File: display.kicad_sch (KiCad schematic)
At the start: 53 parts, among them Q3 SSM6N35AFE, Q4 SSM6N35AFE

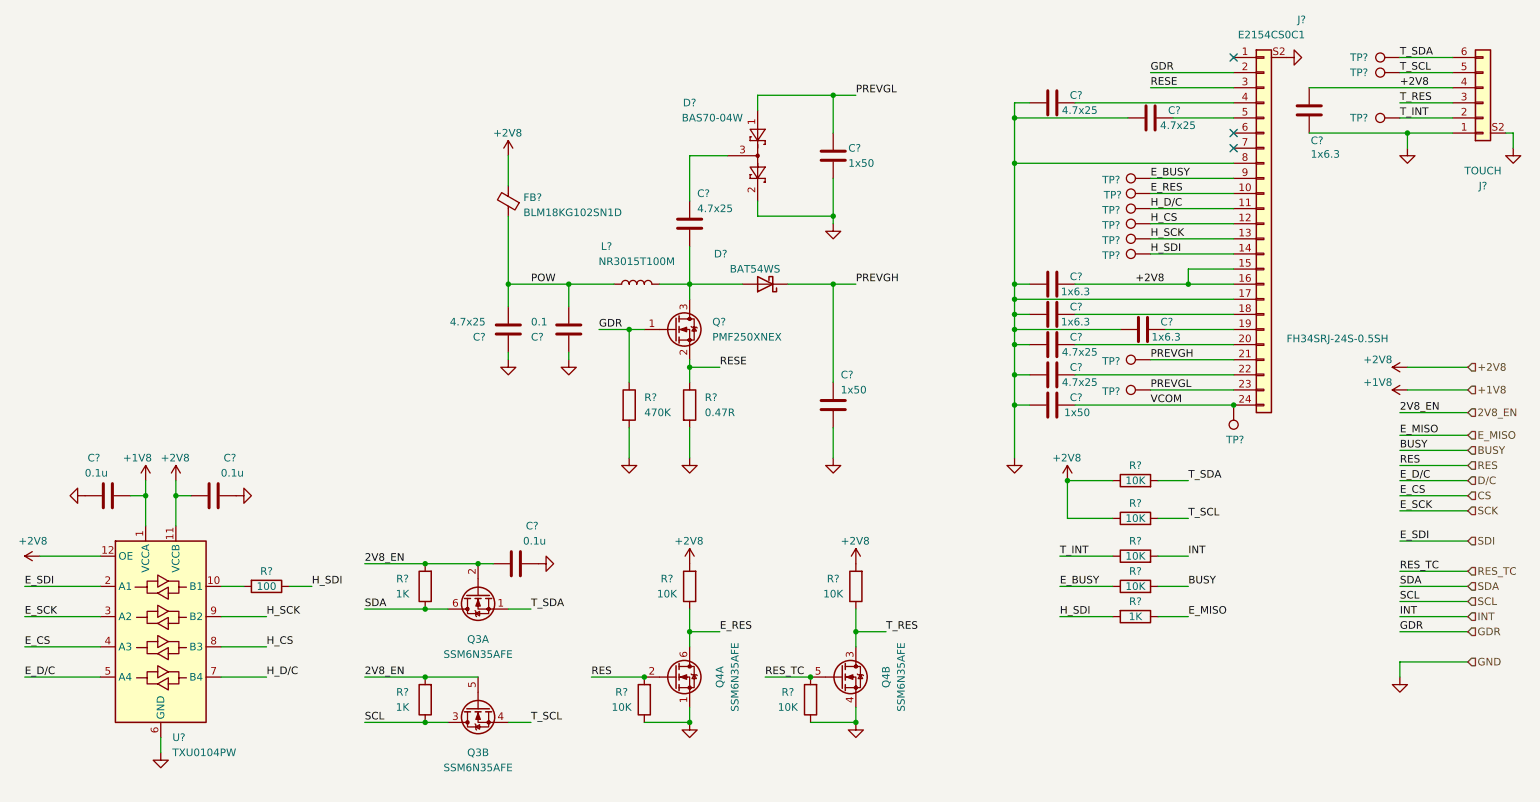
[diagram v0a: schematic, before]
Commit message: Next revision
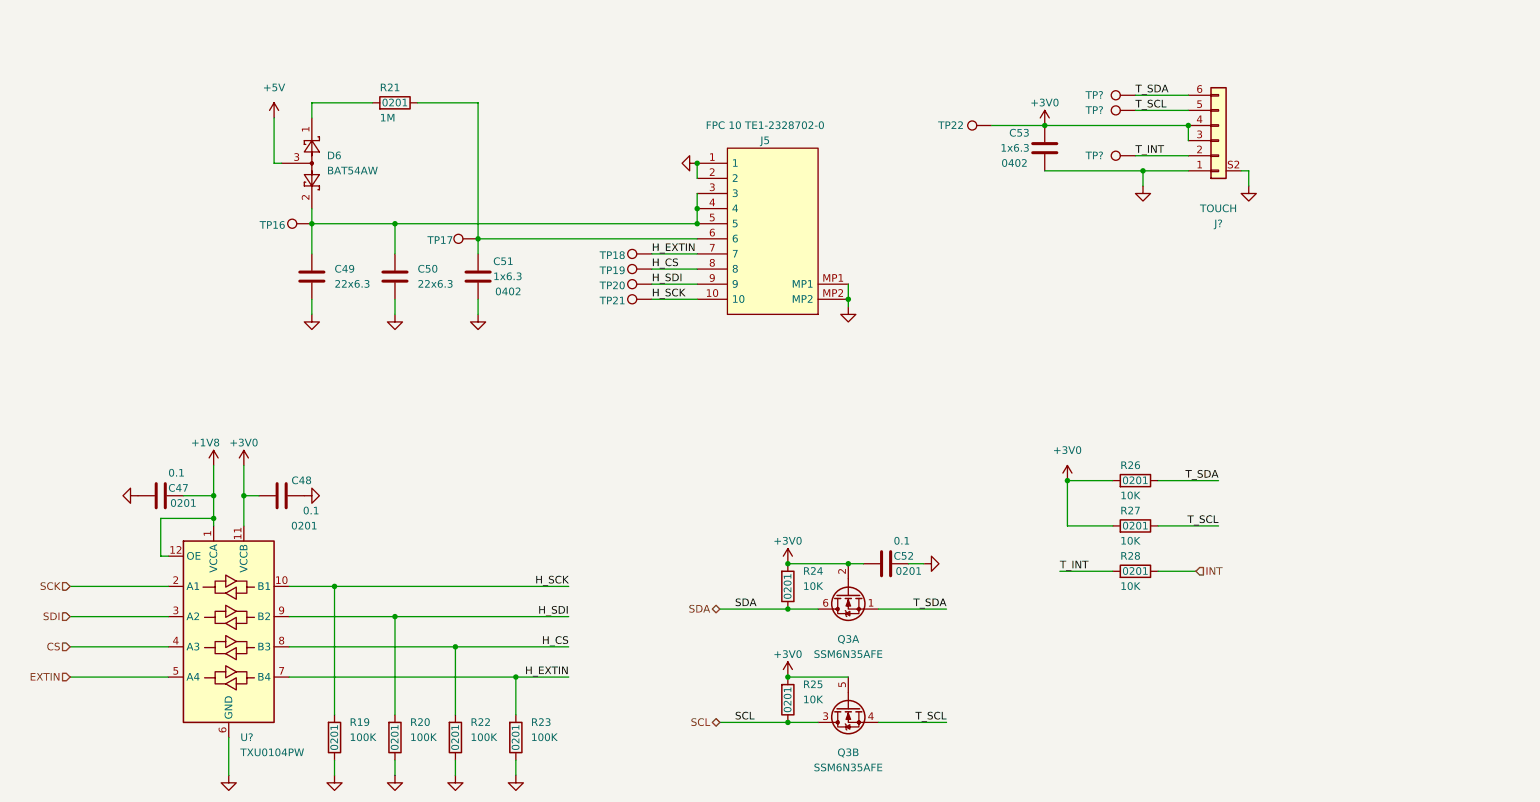
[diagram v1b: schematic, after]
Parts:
- removed C? (x4): 1x6.3, Capacitor_SMD:C_0402_1005Metric, symbol Device:C
- removed C? (x6): 4.7x25, Capacitor_SMD:C_0603_1608Metric, symbol Device:C
- removed C? (x3): 1x50, Capacitor_SMD:C_0402_1005Metric, symbol Device:C
- removed C?: 0.1, Capacitor_SMD:C_0402_1005Metric, symbol Device:C
- removed C? (x3): 0.1u, Capacitor_SMD:C_0402_1005Metric, symbol Device:C
- removed D?: BAT54WS, Diode_SMD:D_SOD-323F, symbol Device:D_Schottky
- removed D?: BAS70-04W, Package_TO_SOT_SMD:SOT-323_SC-70, symbol Diode:BAT54SW
- removed FB?: BLM18KG102SN1D, Inductor_SMD:L_0603_1608Metric, symbol Device:FerriteBead_Small
- removed J?: E2154CS0C1, MyLib:GDEY027T91-T01_bended, symbol Connector_Generic:Conn_01x24
- removed L?: NR3015T100M, Inductor_SMD:L_Wuerth_MAPI-3015, symbol Device:L
- removed Q4: SSM6N35AFE, Package_TO_SOT_SMD:SOT-563, symbol Transistor_FET:FDG1024NZ
- removed Q?: PMF250XNEX, Package_TO_SOT_SMD:SOT-323_SC-70, symbol Device:Q_NMOS_GSD
- removed R? (x8): 10K, Resistor_SMD:R_0402_1005Metric, symbol Device:R
- removed R? (x3): 1K, Resistor_SMD:R_0402_1005Metric, symbol Device:R
- removed R?: 470K, Resistor_SMD:R_0402_1005Metric, symbol Device:R
- removed R?: 100, Resistor_SMD:R_0402_1005Metric, symbol Device:R
- removed R?: 0.47R, Resistor_SMD:R_0603_1608Metric, symbol Device:R
- removed TP? (x9): TestPoint, TestPoint:TestPoint_Pad_D1.0mm, symbol Connector:TestPoint
- added C47, C48, C52: 0.1, Capacitor_SMD:C_0201_0603Metric, symbol Device:C
- added C49, C50: 22x6.3, Capacitor_SMD:C_0603_1608Metric, symbol Device:C
- added C51, C53: 1x6.3, Capacitor_SMD:C_0402_1005Metric, symbol Device:C
- added D6: BAT54AW, MyLib:SOT-523, symbol Diode:BAT54AW
- added J5: FPC 10 TE1-2328702-0, MyLib:TE_123287020, symbol MyLib:FPC 10 TE1-2328702-0
- added R19, R20, R22, R23: 100K, Resistor_SMD:R_0201_0603Metric, symbol Device:R
- added R21: 1M, Resistor_SMD:R_0201_0603Metric, symbol Device:R
- added R24, R25, R26, R27, R28: 10K, Resistor_SMD:R_0201_0603Metric, symbol Device:R
- added TP16, TP17, TP18, TP19, TP20, TP21, TP22: TestPoint, TestPoint:TestPoint_Pad_D1.0mm, symbol Connector:TestPoint
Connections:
- net 2V8_EN is gone; now on net +3V0: Q3.2 (G), Q3.5 (G)
- net T_RES is gone; now on net +3V0: J?.3 (Pin_3)
- net +1V8: now also U?.12 (OE), C47.1
- net GND: now also C47.2, C48.2, C49.1, C50.1, C51.2, C52.1, C53.2, J5.1, J5.2, J5.MP1, J5.MP2, R19.1, R20.1, R22.1, R23.1
- net H_CS: now also J5.8, R22.2, TP19.1
- net H_SCK: now also U?.10 (B1), J5.10, R19.2, TP21.1; no longer U?.9 (B2)
- net H_SDI: now also U?.9 (B2), J5.9, R20.2, TP20.1
- net INT: now also R28.1
- net SCK: now also U?.2 (A1); no longer U?.3 (A2)
- net SCL: now also R25.1
- net SDA: now also R24.1
- net SDI: now also U?.3 (A2); no longer U?.2 (A1)
- net T_INT: now also R28.2
- net T_SCL: now also R27.1
- net T_SDA: now also R26.1
- net +2V8 renamed +3V0
- net +3V0: now also C48.1, C52.2, C53.1, R24.2, R25.2, R26.2, R27.2, TP22.1; no longer U?.12 (OE)
- net D/C renamed EXTIN
- net H_D/C renamed H_EXTIN
- net H_EXTIN: now also J5.7, R23.2, TP18.1
- new net: C51.1, J5.6, R21.1, TP17.1
- new net: C49.2, C50.2, D6.2, J5.3, J5.4, J5.5, TP16.1
- new net: D6.1, R21.2
- new net +5V: D6.3
- no-connect marks 3 -> 0
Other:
- note removed: "FH34SRJ-24S-0.5SH"
- moved on the sheet: J?, Q3A, Q3B, TP?, U?
